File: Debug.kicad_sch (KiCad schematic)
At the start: 11 parts, among them J7 Conn_01x04_Socket, P2 USB_C_Plug_USB2.0

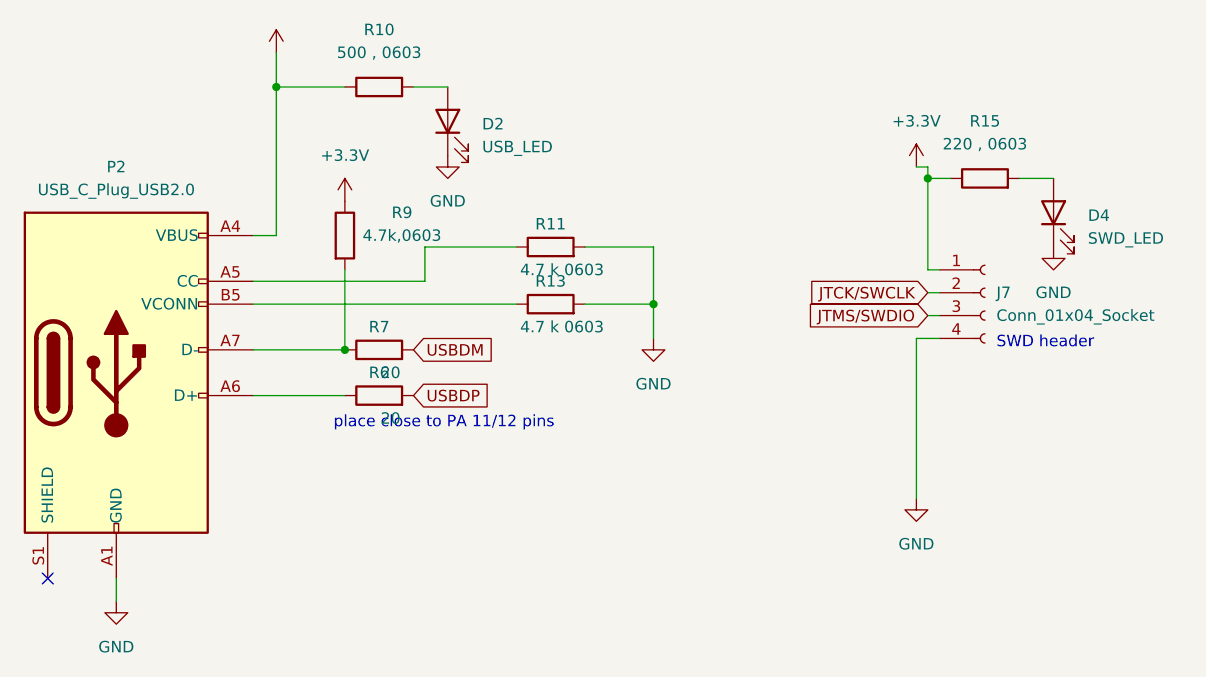
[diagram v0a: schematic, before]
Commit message: Add files via upload
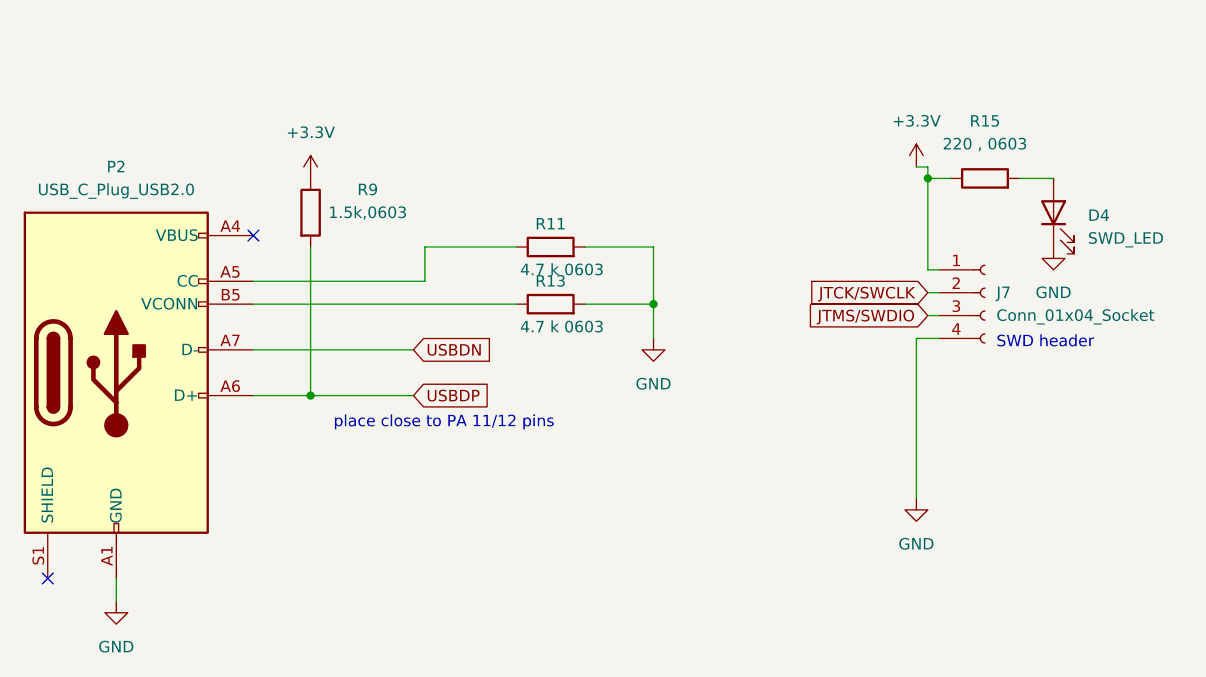
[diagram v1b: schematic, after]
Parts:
- removed D2: USB_LED, LED_SMD:LED_0201_0603Metric, symbol Device:LED
- removed R10: 500 , 0603, Resistor_SMD:R_0201_0603Metric, symbol Device:R
- removed R6, R7: 20, Resistor_SMD:R_0201_0603Metric, symbol Device:R
- P2: footprint Connector_USB:USB_C_Receptacle_Amphenol_12401548E4-2A -> Connector_USB:USB_C_Receptacle_GCT_USB4105-xx-A_16P_TopMnt_Horizontal
- R9: value 4.7k,0603 -> 1.5k,0603
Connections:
- net USBDP: now also P2.A6 (D+), R9.2
- net USBDN: now reaches P2.A7 (D-)
- net USBDN: no longer R9.2
- net +5V: no longer names the net of P2.A4 (VBUS), P2.A9 (VBUS), P2.B4 (VBUS), P2.B9 (VBUS)
- no-connect marks 1 -> 2
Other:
- moved on the sheet: R9
